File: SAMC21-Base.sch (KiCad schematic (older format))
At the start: 63 parts, among them J1 Conn_01x04, J2 Conn_01x10, J3 Conn_01x10, J5 Conn_ARM_JTAG_SWD_10, U1 ATSAMC21E18A-AUT, U2 TJA1043T, U3 LMR50410-Q1, U4 MCP1703A, Y1 8MHz

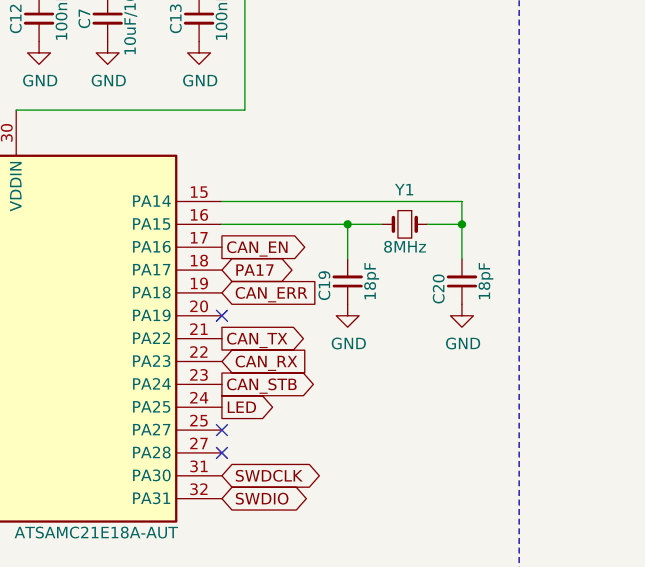
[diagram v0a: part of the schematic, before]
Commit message: cleanup after review-3
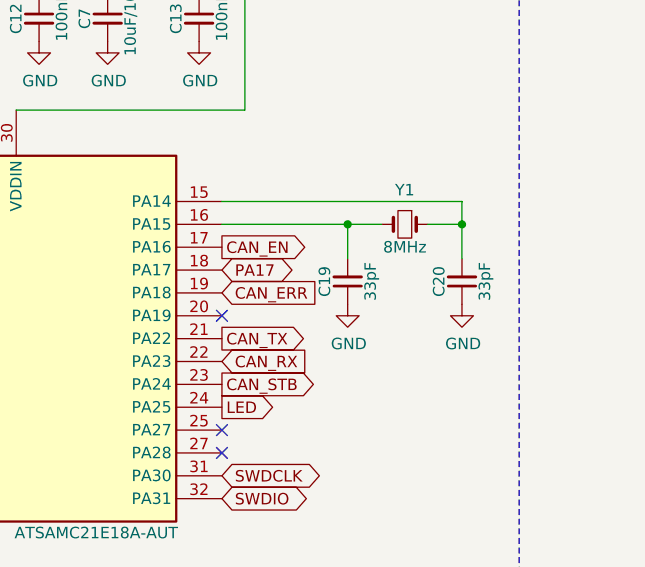
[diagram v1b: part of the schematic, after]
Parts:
- C19, C20: value 18pF -> 33pF
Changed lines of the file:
@@
 U 1 1 60907F03
 P 10600 4650
-F 0 "C20" V 10700 4750 50  0000 R CNN
-F 1 "18pF" V 10500 4650 50  0000 C CNN
+F 0 "C20" V 10700 4650 50  0000 C CNN
+F 1 "33pF" V 10500 4650 50  0000 C CNN
 F 2 "Capacitor_SMD:C_0603_1608Metric" H 10600 4650 50  0001 C CNN
 F 3 "~" H 10600 4650 50  0001 C CNN
@@
 U 1 1 60909D78
 P 10100 4650
-F 0 "C19" V 10200 4600 50  0000 L CNN
-F 1 "18pF" V 10000 4650 50  0000 C CNN
+F 0 "C19" V 10200 4650 50  0000 C CNN
+F 1 "33pF" V 10000 4650 50  0000 C CNN
 F 2 "Capacitor_SMD:C_0603_1608Metric" H 10100 4650 50  0001 C CNN
 F 3 "~" H 10100 4650 50  0001 C CNN
